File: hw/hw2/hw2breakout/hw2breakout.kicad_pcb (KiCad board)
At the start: 2 copper layers, 41.9 x 23.5 mm, 8 parts, among them J1 Conn_01x03_Pin, J2 Conn_01x03_Pin, J3 Conn_01x03_Pin, U1 PCT2075DP

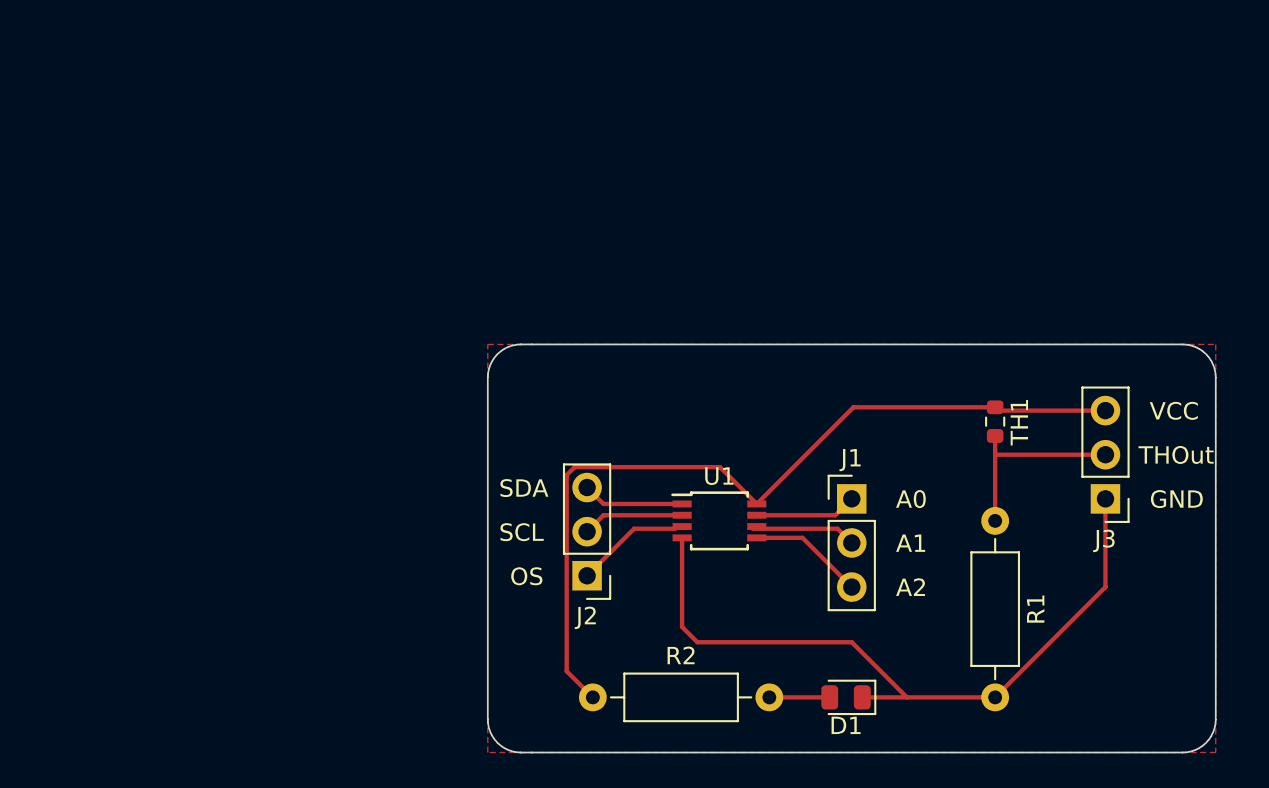
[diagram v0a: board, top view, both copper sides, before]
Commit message: rev 2 for hw2
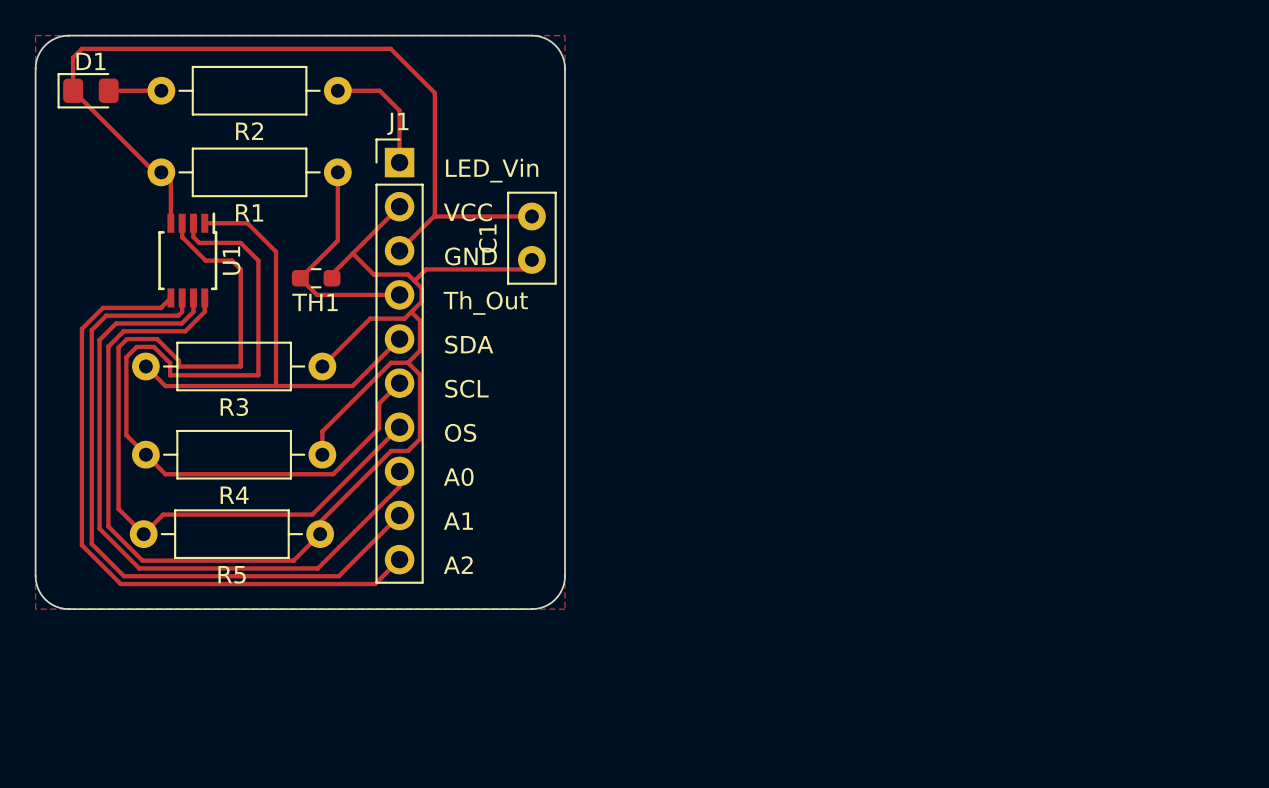
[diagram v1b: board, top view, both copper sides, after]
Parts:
- removed J2, J3: Conn_01x03_Pin, Connector_PinHeader_2.54mm:PinHeader_1x03_P2.54mm_Vertical
- added C1: 0.1uF, Capacitor_THT:C_Disc_D5.0mm_W2.5mm_P2.50mm, F.Cu at (137.2, 54.8)
- added R3: 1.5k, Resistor_THT:R_Axial_DIN0207_L6.3mm_D2.5mm_P10.16mm_Horizontal, F.Cu at (125.1, 61.0)
- added R4: 1.5k, Resistor_THT:R_Axial_DIN0207_L6.3mm_D2.5mm_P10.16mm_Horizontal, F.Cu at (125.1, 66.0)
- added R5: 1.5k, Resistor_THT:R_Axial_DIN0207_L6.3mm_D2.5mm_P10.16mm_Horizontal, F.Cu at (125.0, 70.6)
- D1: footprint LED_SMD:LED_0805_2012Metric -> LED_SMD:LED_0805_2012Metric_Pad1.15x1.40mm_HandSolder
- J1: value Conn_01x03_Pin -> Conn_01x10_Pin; footprint Connector_PinHeader_2.54mm:PinHeader_1x03_P2.54mm_Vertical -> Connector_PinHeader_2.54mm:PinHeader_1x10_P2.54mm_Vertical
- TH1: footprint Resistor_SMD:R_0603_1608Metric -> Resistor_SMD:R_0603_1608Metric_Pad0.98x0.95mm_HandSolder
- moved D1 55.8 mm to (111.8, 45.1), turned to 0 degrees
- moved R1 42.8 mm to (126.0, 49.8), turned to 180 degrees
- moved TH1 40.0 mm to (124.7, 55.9), turned to 180 degrees
- moved R2 37.9 mm to (126.0, 45.1), turned to 180 degrees
- moved U1 34.1 mm to (117.3, 54.9), turned to -90 degrees
- moved J1 32.4 mm to (129.5, 49.2)
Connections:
- J1 pad 1: Net-(J1-Pin_1) -> LED_Vin
- J1 pad 2: Net-(J1-Pin_2) -> VCC
- J1 pad 3: Net-(J1-Pin_3) -> GND
- R1 pad 1: Net-(J3-Pin_2) -> Th_Out
- R2 pad 1: VCC -> LED_Vin
- TH1 pad 2: Net-(J3-Pin_2) -> Th_Out
- U1 pad 1: Net-(J2-Pin_3) -> SDA
- U1 pad 2: Net-(J2-Pin_2) -> SCL
- U1 pad 3: Net-(J2-Pin_1) -> OS
- U1 pad 5: Net-(J1-Pin_3) -> A2
- U1 pad 6: Net-(J1-Pin_2) -> A1
- U1 pad 7: Net-(J1-Pin_1) -> A0
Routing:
- net OS: track 0.00 -> 47.2 mm
- net SCL: track 0.00 -> 44.8 mm
- net A0: track 0.00 -> 38.8 mm
- net A1: track 0.00 -> 38.7 mm
- net A2: track 0.00 -> 38.1 mm
- net VCC: track 47.9 -> 80.7 mm
- net SDA: track 0.00 -> 28.7 mm
- net Th_Out: track 0.00 -> 13.1 mm
- net Net-(J3-Pin_2): track 11.2 -> 0.00 mm
- net GND: track 41.5 -> 49.8 mm
- net LED_Vin: track 0.00 -> 7.02 mm
- net Net-(J1-Pin_3): track 6.64 -> 0.00 mm
- net Net-(J2-Pin_1): track 6.20 -> 0.00 mm
- net Net-(J1-Pin_2): track 6.05 -> 0.00 mm
- net Net-(J1-Pin_1): track 5.86 -> 0.00 mm
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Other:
- board size 41.9 x 23.5 mm -> 30.5 x 33 mm
- board text added: "LED_Vin"
- board text added: "Th_Out"
- board text removed: "THOut"
